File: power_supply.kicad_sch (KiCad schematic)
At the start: 21 parts, among them U3 TPS62913, U4 TPS7A4701RGWR, U5 LDL1117S33R

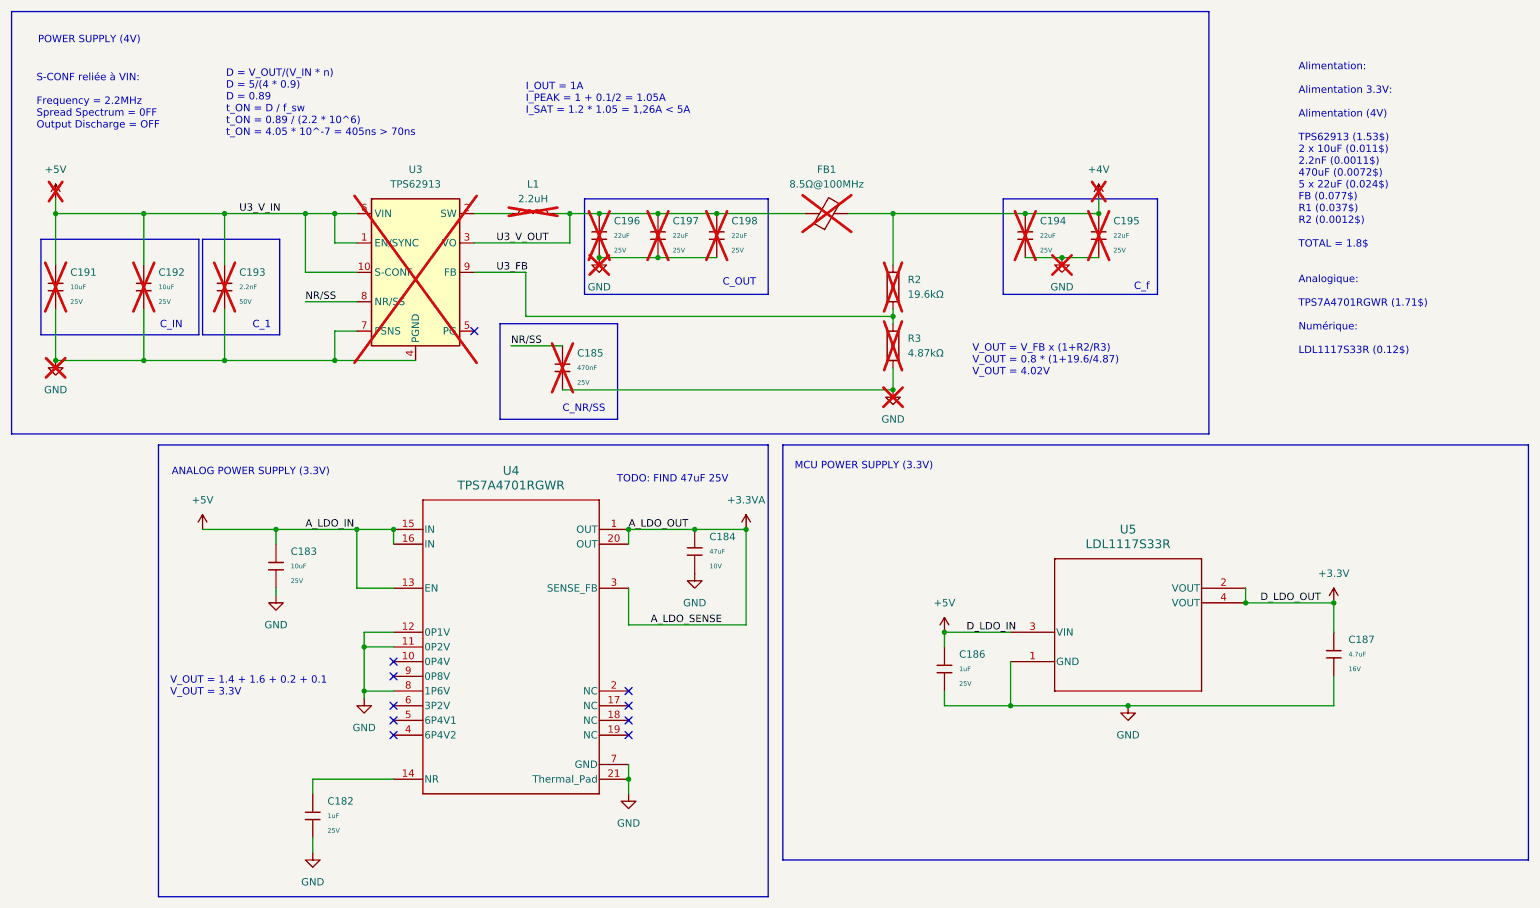
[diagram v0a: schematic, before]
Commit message: caca
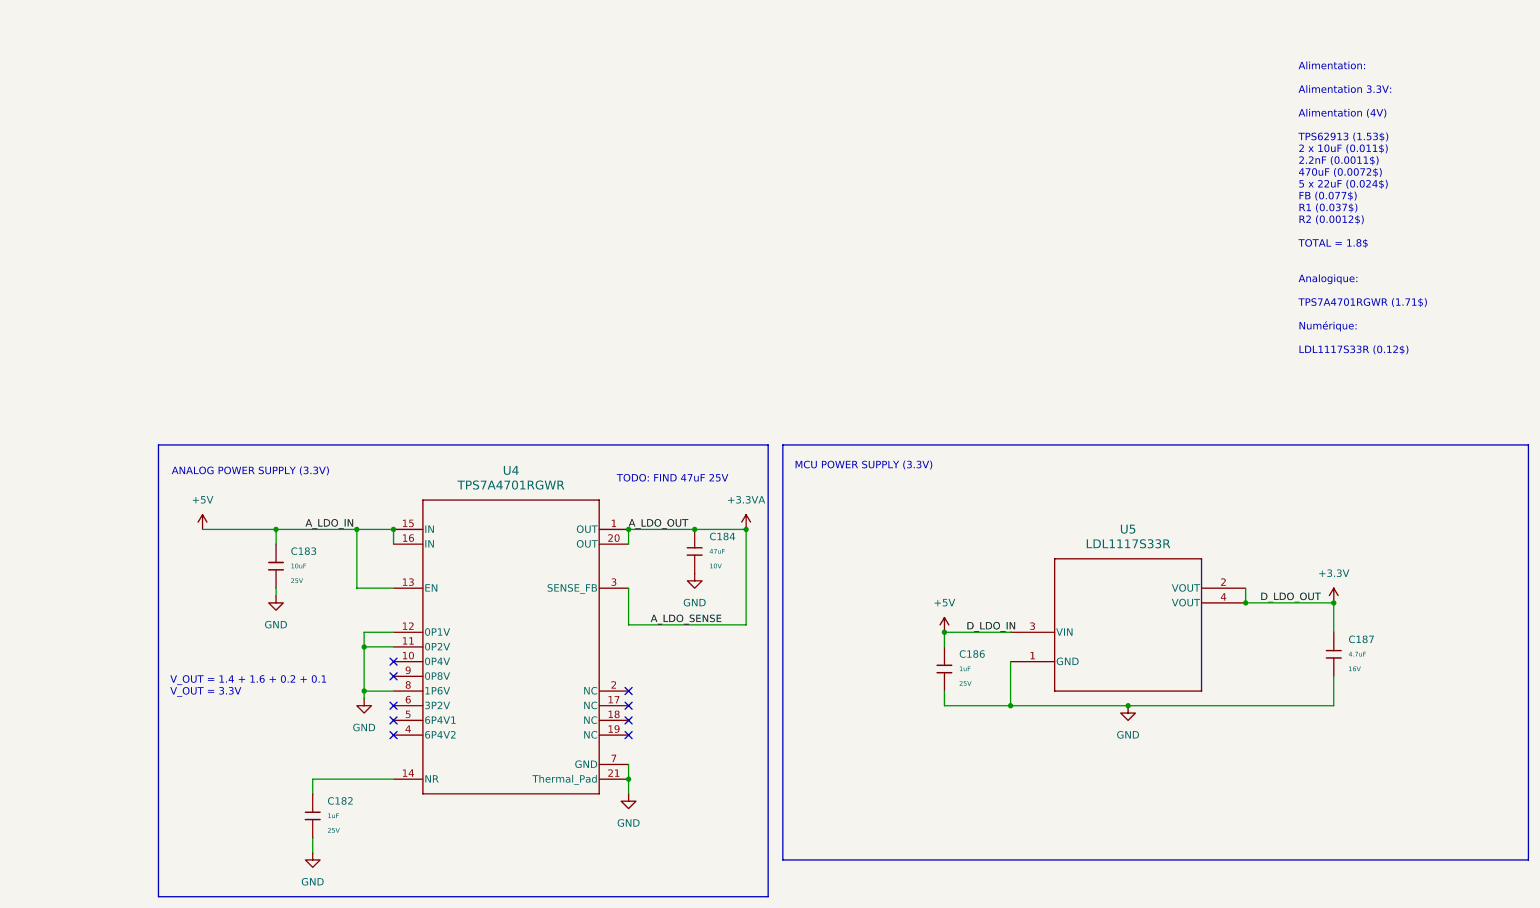
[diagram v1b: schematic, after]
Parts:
- removed C185: 470nF, PCM_JLCPCB:C_0603, symbol PCM_JLCPCB-Capacitors:0603,470nF
- removed C191, C192: 10uF, PCM_JLCPCB:C_0805, symbol PCM_JLCPCB-Capacitors:0805,10uF
- removed C193: 2.2nF, PCM_JLCPCB:C_0402, symbol PCM_JLCPCB-Capacitors:0402,2.2nF
- removed C194, C195, C196, C197, C198: 22uF, PCM_JLCPCB:C_0805, symbol PCM_JLCPCB-Capacitors:0805,22uF
- removed FB1: 8.5Ω@100MHz, PCM_JLCPCB:FB_0603, symbol Device:FerriteBead
- removed L1: 2.2uH, Inductor_SMD:L_1210_3225Metric, symbol Device:L
- removed R2: 19.6kΩ, Resistor_SMD:R_0402_1005Metric, symbol Device:R
- removed R3: 4.87kΩ, PCM_JLCPCB:R_0603, symbol Device:R
- removed U3: TPS62913, Package_DFN_QFN:Texas_RPU0010A_VQFN-HR-10_2x2mm_P0.5mm, symbol Regulator_Switching:TPS62913
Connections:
- no-connect marks 10 -> 9
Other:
- note removed: "C_1"
- note removed: "C_IN"
- note removed: "C_NR/SS"
- note removed: "C_OUT"
- note removed: "C_f"
- note removed: "D = V_OUT/(V_IN * n) D = 5/(4 * 0.9) D = 0.89 t_ON = D / f_sw t_ON = 0.89 / (2.2 * 10^6) t_ON = 4.05 * 10^-7 = 405ns > 70ns"
- note removed: "I_OUT = 1A I_PEAK = 1 + 0.1/2 = 1.05A I_SAT = 1.2 * 1.05 = 1,26A < 5A"
- note removed: "POWER SUPPLY (4V)"
- note removed: "S-CONF reliée à VIN: Frequency = 2.2MHz Spread Spectrum = 0FF Output Discharge = OFF"
- note removed: "V_OUT = V_FB x (1+R2/R3) V_OUT = 0.8 * (1+19.6/4.87) V_OUT = 4.02V"
